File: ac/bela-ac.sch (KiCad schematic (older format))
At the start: 0 parts

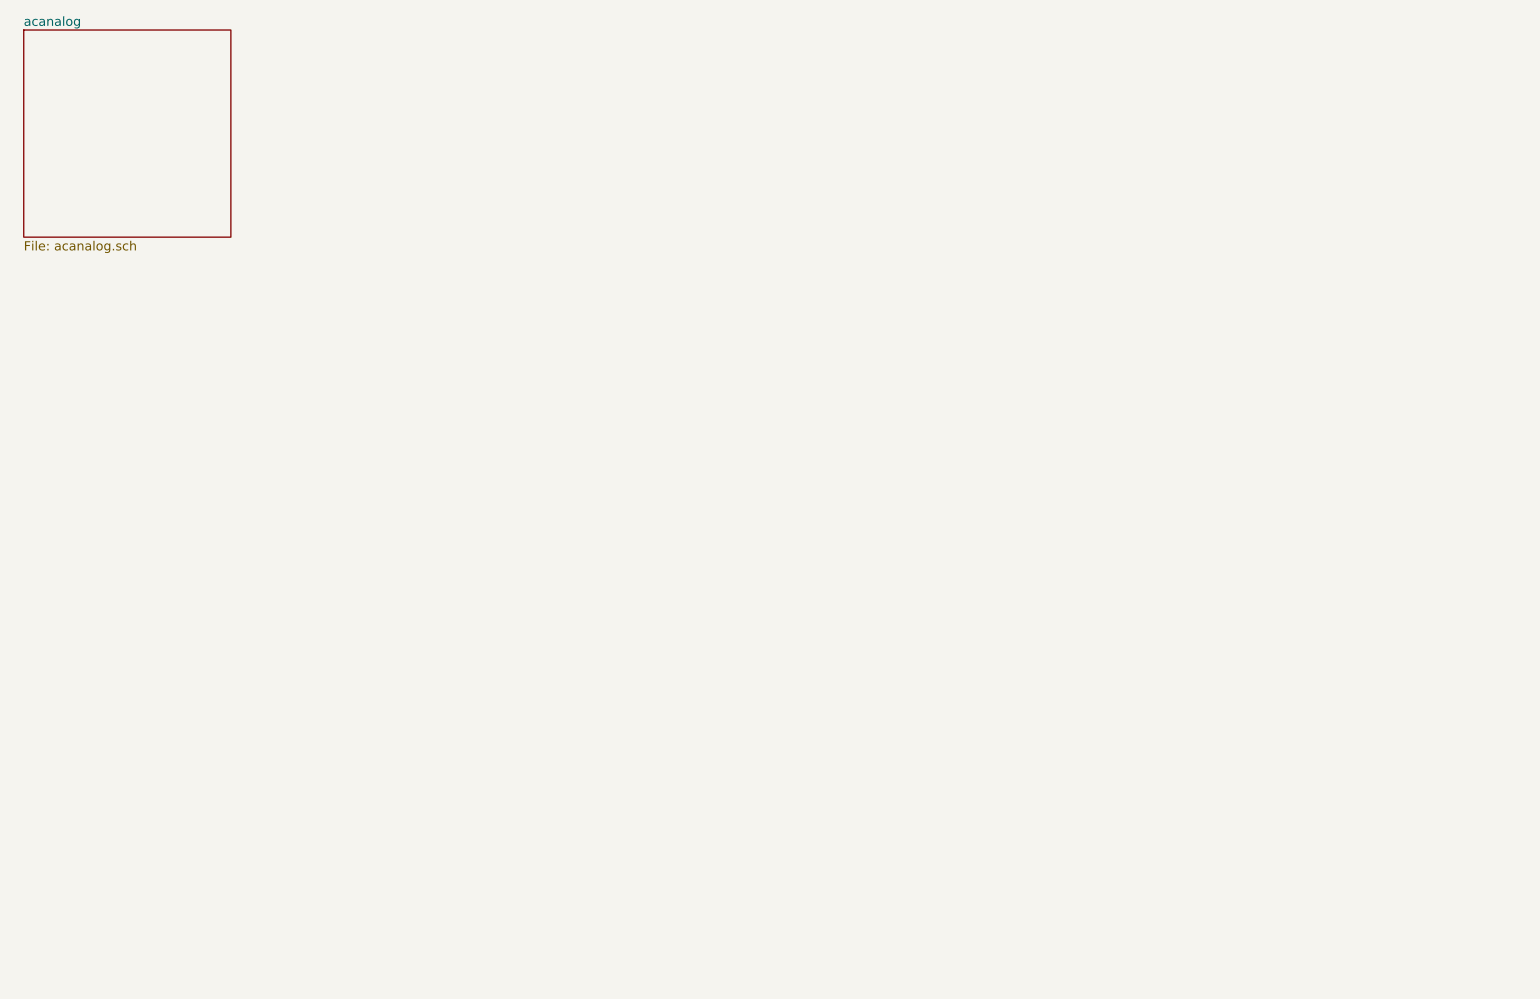
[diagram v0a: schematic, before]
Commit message: consolidated schematics etc
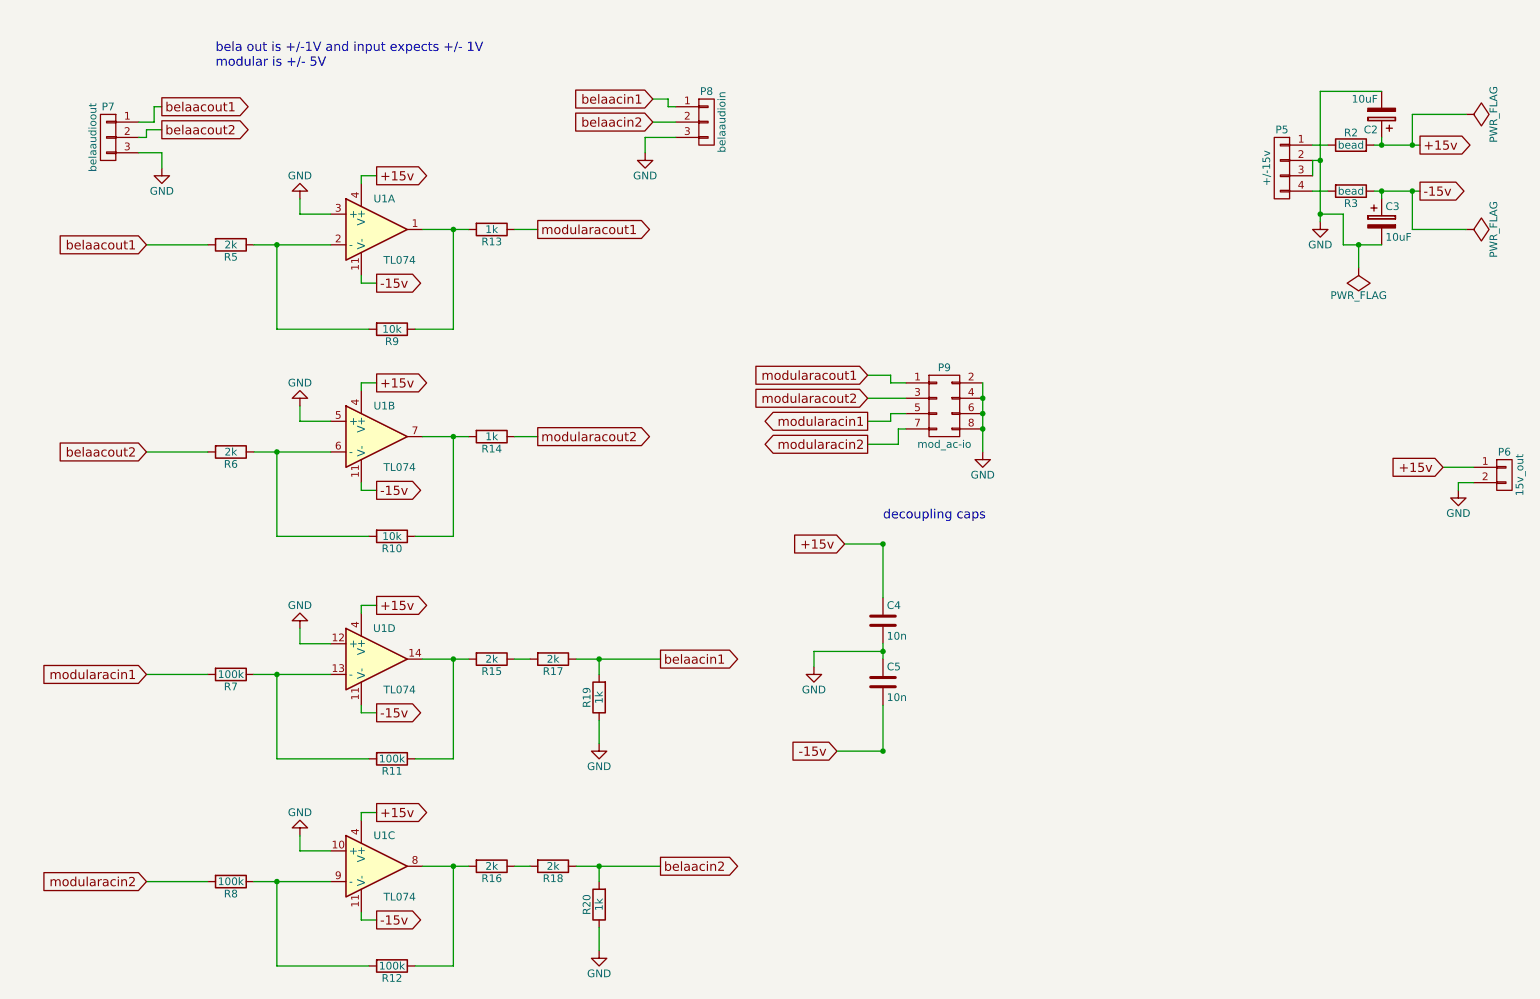
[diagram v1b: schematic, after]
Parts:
- added C2, C3: 10uF, Capacitors_ThroughHole:C_Radial_D5_L11_P2, symbol CP
- added C4, C5: 10n, Capacitors_ThroughHole:C_Rect_L4_W2.5_P2.5, symbol C
- added P5: +/-15v, mta-156:MTA-156-4, symbol MTA-156-4
- added P6: 15v_out, Pin_Headers:Pin_Header_Straight_1x02_Pitch2.54mm, symbol CONN_01X02
- added P7: belaaudioout, Pin_Headers:Pin_Header_Straight_1x03_Pitch2.54mm, symbol CONN_01X03
- added P8: belaaudioin, Pin_Headers:Pin_Header_Straight_1x03_Pitch2.54mm, symbol CONN_01X03
- added P9: mod_ac-io, Pin_Headers:Pin_Header_Straight_2x04_Pitch2.54mm, symbol CONN_02X04
- added R10, R9: 10k, xnorman:Resistor_Horizontal_RM10mm-xnorman, symbol R
- added R11, R12, R7, R8: 100k, xnorman:Resistor_Horizontal_RM10mm-xnorman, symbol R
- added R13, R14, R19, R20: 1k, xnorman:Resistor_Horizontal_RM10mm-xnorman, symbol R
- added R15, R16, R17, R18, R5, R6: 2k, xnorman:Resistor_Horizontal_RM10mm-xnorman, symbol R
- added R2, R3: bead, xnorman:Resistor_Vertical_RM5mm-xnor, symbol R
- added U1: TL074, Housings_DIP:DIP-14_W7.62mm_LongPads, symbol TL074
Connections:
- new net: R13.2, R9.1, U1.1
- new net: R5.1, R9.2, U1.2 (-)
- new net: R10.2, R6.1, U1.6 (-)
- new net: R10.1, R14.2, U1.7
- new net: R11.2, R7.1, U1.13 (-)
- new net: R11.1, R15.2, U1.14
- new net: R15.1, R17.2
- new net: R12.1, R16.2, U1.8
- new net: R12.2, R8.1, U1.9 (-)
- new net: R16.1, R18.2
- new net: P5.1 (P1), R2.1
- new net: P5.4 (P4), R3.2
- new net +15v: C2.1, C4.1, P6.1 (P1), R2.2, U1.4 (V+), U1.4 (V+), U1.4 (V+), U1.4 (V+)
- new net -15v: C3.1, C5.2, R3.1, U1.11 (V-), U1.11 (V-), U1.11 (V-), U1.11 (V-)
- new net GND: C2.2, C3.2, C4.2, C5.1, P5.2 (P2), P5.3 (P3), P6.2 (P2), P7.3 (P3), P8.3 (P3), P9.2 (P2), P9.4 (P4), P9.6 (P6), P9.8 (P8), R19.1, R20.1, U1.10 (+), U1.12 (+), U1.3 (+), U1.5 (+)
- new net belaacin1: P8.1 (P1), R17.1, R19.2
- new net belaacin2: P8.2 (P2), R18.1, R20.2
- new net belaacout1: P7.1 (P1), R5.2
- new net belaacout2: P7.2 (P2), R6.2
- new net modularacin1: P9.5 (P5), R7.2
- new net modularacin2: P9.7 (P7), R8.2
- new net modularacout1: P9.1 (P1), R13.1
- new net modularacout2: P9.3 (P3), R14.1
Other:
- note added: "bela out is +/-1V and input expects +/- 1V\nmodular is +/- 5V"
- note added: "decoupling caps"
